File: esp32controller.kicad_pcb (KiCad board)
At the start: 2 copper layers, 80 x 100 mm, 117 parts, among them J1 Conn_02x03_Odd_Even, J10 USB_B_Micro, J11 Conn_01x04_Female, J12 Conn_01x06_Female, J14 Conn_01x04, J15 Conn_01x06, J16 Conn_01x04, J17 Conn_01x04, J18 Conn_01x03, J19 Conn_01x03, J2 Conn_01x04, J20 Conn_01x03, J21 Conn_02x09_Odd_Even, J22 Conn_02x09_Odd_Even, J23 Conn_01x03, J24 Conn_01x03, J25 Conn_01x03, J26 Conn_02x09_Odd_Even, J3 Conn_02x03_Odd_Even, J4 Conn_01x04, J5 Conn_02x03_Odd_Even, J6 Conn_01x04, J7 Micro_SD_Card_Det, J8 Conn_02x03_Odd_Even, J9 Conn_01x04, Q1 Q_NPN_BEC, Q2 Q_NPN_BEC, Q3 Q_NMOS_GDS, Q4 Q_NMOS_GDS, Q5 Q_NMOS_GDS, U1 ESP32-WROOM, U2 CH340C, U3 ADS1015, U4 SX1509, U5 TPS560430, U6 TLV1117-33

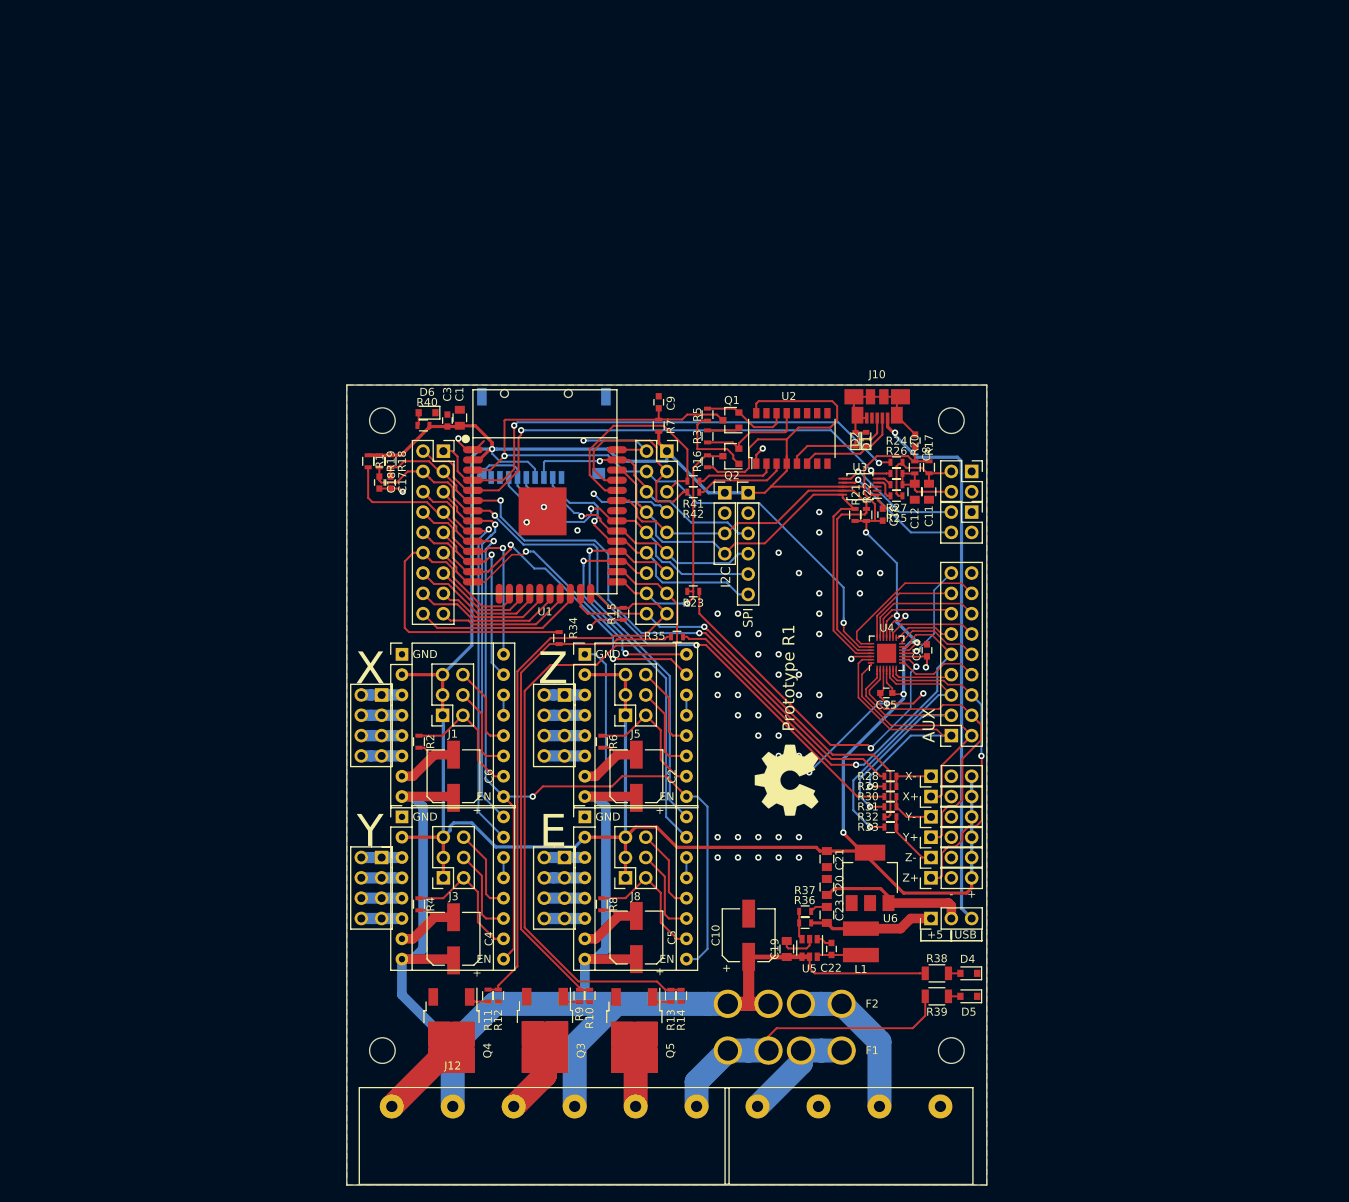
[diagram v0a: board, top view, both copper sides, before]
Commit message: Prototype R2
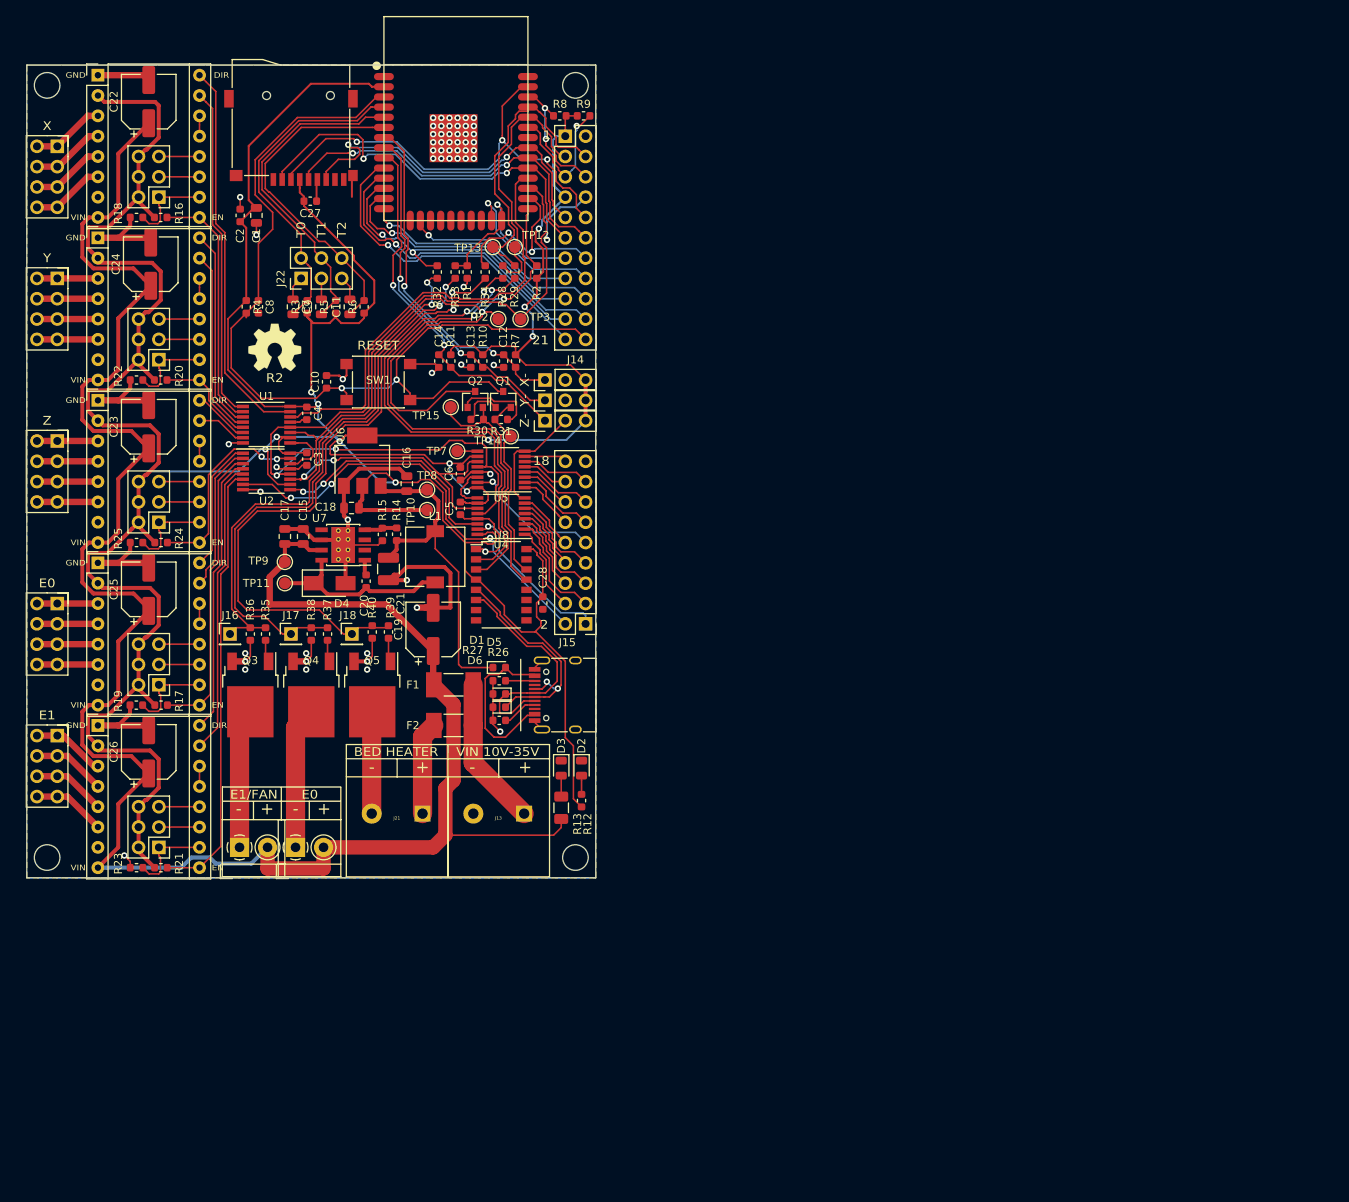
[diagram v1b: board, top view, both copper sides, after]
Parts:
- removed J26: Conn_02x09_Odd_Even, Socket_Strips:Socket_Strip_Straight_2x09_Pitch2.54mm
- removed JP1: Jumper_3_Open, Socket_Strips:Socket_Strip_Straight_1x03_Pitch2.54mm
- removed MK1, MK2, MK3, MK4: Mounting_Hole, Mounting_Holes:MountingHole_3.2mm_M3
- removed R41, R42: 0, Resistors_SMD:R_0603
- removed REF***: OSHW-Symbol_8.9x8mm_SilkScreen, Symbols:OSHW-Symbol_8.9x8mm_SilkScreen
- added A5: Pololu_Breakout_A4988, Module:Pololu_Breakout-16_15.2x20.3mm, F.Cu at (8.89, 82.5)
- added C13: NC, Capacitor_SMD:C_0603_1608Metric, F.Cu at (55.5, 37.0)
- added C24: 100uF, Capacitor_SMD:CP_Elec_6.3x7.7, F.Cu at (15.5, 24.9)
- added C25: 100uF, Capacitor_SMD:CP_Elec_6.3x7.7, F.Cu at (15.2, 65.5)
- added C26: 100uF, Capacitor_SMD:CP_Elec_6.3x7.7, F.Cu at (15.2, 85.9)
- added C27: 100nF, Capacitor_SMD:C_0603_1608Metric, F.Cu at (35.4, 17.0)
- added C28: 100nF, Capacitor_SMD:C_0603_1608Metric, F.Cu at (64.5, 67.2)
- added C7: 10uF, Capacitor_SMD:C_0805_2012Metric, F.Cu at (33.3, 30.2)
- added D3: LED, LED_SMD:LED_0805_2012Metric, F.Cu at (66.8, 87.9)
- added J13: Conn_01x02, ESP32-footprints-Lib:TERM_2-WAY_6.35mm, F.Cu at (59.0, 93.6)
- added REF**: OSHW-Symbol_6.7x6mm_SilkScreen, Symbol:OSHW-Symbol_6.7x6mm_SilkScreen, F.Cu at (31.0, 35.3)
- added REF**: MountingHole_3.2mm_M3_DIN965, MountingHole:MountingHole_3.2mm_M3_DIN965, F.Cu at (68.6, 2.54)
- added REF**: MountingHole_3.2mm_M3_DIN965, MountingHole:MountingHole_3.2mm_M3_DIN965, F.Cu at (2.54, 2.54)
- added REF**: MountingHole_3.2mm_M3_DIN965, MountingHole:MountingHole_3.2mm_M3_DIN965, F.Cu at (2.54, 99.1)
- added REF**: MountingHole_3.2mm_M3_DIN965, MountingHole:MountingHole_3.2mm_M3_DIN965, F.Cu at (68.6, 99.1)
- added SW1: SW_Push, Button_Switch_SMD:SW_Push_1P1T_NO_6x6mm_H9.5mm, F.Cu at (43.9, 39.6)
- added TP10: TestPoint, TestPoint:TestPoint_Pad_D1.5mm, F.Cu at (50.0, 55.6)
- added TP11: TestPoint, TestPoint:TestPoint_Pad_D1.5mm, F.Cu at (32.3, 64.8)
- added TP12: TestPoint, TestPoint:TestPoint_Pad_D1.5mm, F.Cu at (61.0, 22.8)
- added TP13: TestPoint, TestPoint:TestPoint_Pad_D1.5mm, F.Cu at (58.2, 22.8)
- added TP14: TestPoint, TestPoint:TestPoint_Pad_D1.5mm, F.Cu at (60.5, 46.4)
- added TP15: TestPoint, TestPoint:TestPoint_Pad_D1.5mm, F.Cu at (53.0, 42.8)
- added TP2: TestPoint, TestPoint:TestPoint_Pad_D1.5mm, F.Cu at (58.9, 31.8)
- added TP3: TestPoint, TestPoint:TestPoint_Pad_D1.5mm, F.Cu at (61.7, 31.8)
- added TP7: TestPoint, TestPoint:TestPoint_Pad_D1.5mm, F.Cu at (53.8, 48.3)
- added TP8: TestPoint, TestPoint:TestPoint_Pad_D1.5mm, F.Cu at (50.0, 53.1)
- added TP9: TestPoint, TestPoint:TestPoint_Pad_D1.5mm, F.Cu at (32.3, 62.1)
- added U7: TPS5430DDA, Package_SO:TI_SO-PowerPAD-8_ThermalVias, F.Cu at (39.5, 60.0)
- added U8: CH340C, Package_SO:SOP-16_4.4x10.4mm_P1.27mm, F.Cu at (59.3, 65.0)
- C1: value 100uF -> 10uF; footprint Capacitors_SMD:C_0805 -> Capacitor_SMD:C_0805_2012Metric
- C10, C4, C5, C6: value 100uF -> 100nF; footprint Capacitors_SMD:CP_Elec_6.3x7.7 -> Capacitor_SMD:C_0603_1608Metric
- C11: footprint Capacitors_SMD:C_0805 -> Capacitor_SMD:C_0805_2012Metric
- C12: value 10uF -> NC; footprint Capacitors_SMD:C_0805 -> Capacitor_SMD:C_0603_1608Metric
- C14: value 100nF -> NC; footprint Capacitors_SMD:C_0603 -> Capacitor_SMD:C_0603_1608Metric
- C15: value 100nF -> 4.7uF; footprint Capacitors_SMD:C_0603 -> Capacitor_SMD:C_0805_2012Metric
- C16: value 100n -> 10uF; footprint Capacitors_SMD:C_0603 -> Capacitor_SMD:C_0805_2012Metric
- C17: value NC -> 4.7uF; footprint Capacitors_SMD:C_0603 -> Capacitor_SMD:C_0805_2012Metric
- C18: value NC -> 10uF; footprint Capacitors_SMD:C_0603 -> Capacitor_SMD:C_0805_2012Metric
- C19: value 2.2uF -> 100uF; footprint Capacitors_SMD:C_0805 -> Capacitor_SMD:CP_Elec_6.3x7.7
- C2: value 100uF -> 1uF; footprint Capacitors_SMD:CP_Elec_6.3x7.7 -> Capacitor_SMD:C_0603_1608Metric
- C20: value 10uF -> 10nF; footprint Capacitors_SMD:C_0805 -> Capacitor_SMD:C_0603_1608Metric
- C21: value 100uF -> 220uF; footprint Capacitors_SMD:C_0805 -> Capacitor_SMD:C_1210_3225Metric
- C22: value 0.1uF -> 100uF; footprint Capacitors_SMD:C_0603 -> Capacitor_SMD:CP_Elec_6.3x7.7
- C23: value 22uF -> 100uF; footprint Capacitors_SMD:C_0805 -> Capacitor_SMD:CP_Elec_6.3x7.7
- C3: value 1uF -> 100nF; footprint Capacitors_SMD:C_0603 -> Capacitor_SMD:C_0603_1608Metric
- C8: value 100n -> 100nF; footprint Capacitors_SMD:C_0603 -> Capacitor_SMD:C_0603_1608Metric
- C9: value 1nF -> 10uF; footprint Capacitors_SMD:C_0603 -> Capacitor_SMD:C_0805_2012Metric
- D1: value D_TVS -> D_Schottky; footprint Diodes_SMD:D_0603 -> Diode_SMD:D_0603_1608Metric
- D2: value D_TVS -> LED; footprint Diodes_SMD:D_0603 -> LED_SMD:LED_0805_2012Metric
- D4: value LED -> B340A; footprint Diodes_SMD:D_0805 -> Diode_SMD:D_SMA
- D5, D6: value LED -> D_TVS; footprint Diodes_SMD:D_0805 -> Diode_SMD:D_0603_1608Metric
- F1, F2: footprint ESP32Controller:FUSE -> ESP32Controller:Fuse_0679H
- J1, J5: footprint Socket_Strips:Socket_Strip_Straight_2x03_Pitch2.54mm -> Connector_PinHeader_2.54mm:PinHeader_2x03_P2.54mm_Vertical
- J10: value USB_B_Micro -> Conn_01x04; footprint ESP32Controller:473460001 -> ESP32Controller:Socket_Strip_Straight_1x04_Pitch2.54mm_dual
- J11: value Conn_01x04_Female -> Micro_SD_Card_Det; footprint ESP32Controller:KP7.62x4 -> ESP32Controller:microsd
- J12: value Conn_01x06_Female -> USB_C_Receptacle_USB2.0; footprint ESP32Controller:KP7.62x6 -> ESP32Controller:USB_C
- J14: value Conn_01x04 -> Conn_02x11_Odd_Even; footprint Socket_Strips:Socket_Strip_Straight_1x04_Pitch2.54mm -> Connector_PinHeader_2.54mm:PinHeader_2x11_P2.54mm_Vertical
- J15: value Conn_01x06 -> Conn_02x09_Odd_Even; footprint Socket_Strips:Socket_Strip_Straight_1x06_Pitch2.54mm -> Connector_PinHeader_2.54mm:PinHeader_2x09_P2.54mm_Vertical
- J16, J17: value Conn_01x04 -> Conn_01x01; footprint Socket_Strips:Socket_Strip_Straight_2x02_Pitch2.54mm -> Connector_PinHeader_2.54mm:PinHeader_1x01_P2.54mm_Vertical
- J18: value Conn_01x03 -> Conn_01x01; footprint Socket_Strips:Socket_Strip_Straight_1x03_Pitch2.54mm -> Connector_PinHeader_2.54mm:PinHeader_1x01_P2.54mm_Vertical
- J19, J20: value Conn_01x03 -> Conn_01x02; footprint Socket_Strips:Socket_Strip_Straight_1x03_Pitch2.54mm -> TerminalBlock_4Ucon:TerminalBlock_4Ucon_1x02_P3.50mm_Horizontal
- J2, J6, J9: value Conn_01x04 -> Conn_02x03_Odd_Even; footprint ESP32Controller:Socket_Strip_Straight_1x04_Pitch2.54mm_dual -> Connector_PinHeader_2.54mm:PinHeader_2x03_P2.54mm_Vertical
- J21: value Conn_02x09_Odd_Even -> Conn_01x02; footprint Socket_Strips:Socket_Strip_Straight_2x09_Pitch2.54mm -> ESP32-footprints-Lib:TERM_2-WAY_6.35mm
- J22: value Conn_02x09_Odd_Even -> Conn_01x06; footprint Socket_Strips:Socket_Strip_Straight_2x09_Pitch2.54mm -> Connector_PinHeader_2.54mm:PinHeader_2x03_P2.54mm_Vertical
- J23, J24, J25: footprint Socket_Strips:Socket_Strip_Straight_1x03_Pitch2.54mm -> Connector_PinHeader_2.54mm:PinHeader_1x03_P2.54mm_Vertical
- J3, J8: value Conn_02x03_Odd_Even -> Conn_01x04; footprint Socket_Strips:Socket_Strip_Straight_2x03_Pitch2.54mm -> ESP32Controller:Socket_Strip_Straight_1x04_Pitch2.54mm_dual
- J7: value Micro_SD_Card_Det -> Conn_01x04; footprint ESP32Controller:microsd -> ESP32Controller:Socket_Strip_Straight_1x04_Pitch2.54mm_dual; moved to F.Cu
- L1: value 18uH -> 22uH; footprint ESP32Controller:SDR0403 -> Inductor_SMD:L_7.3x7.3_H3.5
- Q1, Q2: footprint TO_SOT_Packages_SMD:SOT-23 -> Package_TO_SOT_SMD:SOT-23
- Q3, Q4, Q5: footprint TO_SOT_Packages_SMD:TO-252-2 -> Package_TO_SOT_SMD:TO-252-2
- R1: value 10k -> DNP 10k; footprint Resistors_SMD:R_0603 -> Resistor_SMD:R_0603_1608Metric
- R10, R14, R2, R4: value 100k -> 10k; footprint Resistors_SMD:R_0603 -> Resistor_SMD:R_0603_1608Metric
- R11: value 10 -> 10k; footprint Resistors_SMD:R_0603 -> Resistor_SMD:R_0603_1608Metric
- R12: value 100k -> R; footprint Resistors_SMD:R_0603 -> Resistor_SMD:R_0603_1608Metric
- R13: value 10 -> 2.4k; footprint Resistors_SMD:R_0603 -> Resistor_SMD:R_1206_3216Metric
- R15: value 5k -> 3.24k; footprint Resistors_SMD:R_0603 -> Resistor_SMD:R_0603_1608Metric
- R16: value 5k -> 10k; footprint Resistors_SMD:R_0603 -> Resistor_SMD:R_0603_1608Metric
- R17, R20, R21: value 4.7k -> 10k; footprint Resistors_SMD:R_0603 -> Resistor_SMD:R_0603_1608Metric
- R18, R19: value 10k -> 100k; footprint Resistors_SMD:R_0603 -> Resistor_SMD:R_0603_1608Metric
- R22: value 4.7k -> 100k; footprint Resistors_SMD:R_0603 -> Resistor_SMD:R_0603_1608Metric
- R23, R25: value 0 -> 100k; footprint Resistors_SMD:R_0603 -> Resistor_SMD:R_0603_1608Metric
- R24, R30, R31: value 0 -> 10k; footprint Resistors_SMD:R_0603 -> Resistor_SMD:R_0603_1608Metric
- R26, R27: value 0 -> 5.1k; footprint Resistors_SMD:R_0603 -> Resistor_SMD:R_0603_1608Metric
- R28, R32, R33, R34: footprint Resistors_SMD:R_0603 -> Resistor_SMD:R_0603_1608Metric
- R29: value 0 -> 499; footprint Resistors_SMD:R_0603 -> Resistor_SMD:R_0603_1608Metric
- R3, R5: value 12k -> 4.7k; footprint Resistors_SMD:R_0603 -> Resistor_SMD:R_0603_1608Metric
- R35: value 0 -> 10; footprint Resistors_SMD:R_0603 -> Resistor_SMD:R_0603_1608Metric
- R36: value 88.7k -> 100k; footprint Resistors_SMD:R_0603 -> Resistor_SMD:R_0603_1608Metric
- R37: value 22.1k -> 10; footprint Resistors_SMD:R_0603 -> Resistor_SMD:R_0603_1608Metric
- R38: value 1.5k -> 100k; footprint Resistors_SMD:R_1206 -> Resistor_SMD:R_0603_1608Metric
- R39: value 1.5k -> 10; footprint Resistors_SMD:R_1206 -> Resistor_SMD:R_0603_1608Metric
- R40: value R -> 100k; footprint Resistors_SMD:R_0603 -> Resistor_SMD:R_0603_1608Metric
- R6, R8: value 100k -> 4.7k; footprint Resistors_SMD:R_0603 -> Resistor_SMD:R_0603_1608Metric
- R7: value 12k -> 10k; footprint Resistors_SMD:R_0603 -> Resistor_SMD:R_0603_1608Metric
- R9: value 10 -> 4.7k; footprint Resistors_SMD:R_0603 -> Resistor_SMD:R_0603_1608Metric
- U1: value ESP32-WROOM -> 74HC595; footprint ESP32-footprints-Lib:ESP32-WROOM -> Package_SO:TSSOP-16_4.4x5mm_P0.65mm
- U2: value CH340C -> 74HC595; footprint Housings_SSOP:SOP-16_4.4x10.4mm_Pitch1.27mm -> Package_SO:TSSOP-16_4.4x5mm_P0.65mm
- U3: value ADS1015 -> ESP32-WROOM; footprint Housings_SSOP:TSSOP-10_3x3mm_Pitch0.5mm -> ESP32-footprints-Lib:ESP32-WROOM
- U4: value SX1509 -> 74HC595; footprint Housings_DFN_QFN:QFN-28-1EP_4x4mm_Pitch0.4mm -> Package_SO:TSSOP-16_4.4x5mm_P0.65mm
- U5: value TPS560430 -> 74HC595; footprint TO_SOT_Packages_SMD:SOT-23-6 -> Package_SO:TSSOP-16_4.4x5mm_P0.65mm
- U6: footprint TO_SOT_Packages_SMD:SOT-223-3_TabPin2 -> Package_TO_SOT_SMD:SOT-223-3_TabPin2
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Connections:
- A1 pad 15: /IO27 -> Q1
- A1 pad 16: /IO26 -> Q0
- A1 pad 2: VCC -> +3.3V
- A1 pad 8: +24V -> VIN_FUSED
- A1 pad 9: /IO25 -> Q2
- A2 pad 15: /IO33 -> Q4
- A2 pad 16: /IO32 -> Q3
- A2 pad 2: VCC -> +3.3V
- A2 pad 8: +24V -> VIN_FUSED
- A2 pad 9: /IO25 -> Q5
- A3 pad 15: /IO14 -> Q7
- A3 pad 16: /IO12 -> Q6
- A3 pad 2: VCC -> +3.3V
- A3 pad 8: +24V -> VIN_FUSED
- A3 pad 9: /IO25 -> Q8
- A4 pad 15: /E0_STEP -> Q10
- A4 pad 16: /E0_DIR -> Q9
- A4 pad 2: VCC -> +3.3V
- A4 pad 8: +24V -> VIN_FUSED
- A4 pad 9: /IO25 -> Q11
- C1 pad 1: VCC -> +3.3V
- C10 pad 1: +24V -> EN
- C11 pad 1: /THERM0 -> THERM2
- C12 pad 1: /THERM1 -> X_MIN
- C14 pad 1: VCC -> Z_MIN
- C15 pad 1: VCC -> VIN_FUSED
- C16 pad 1: VCC -> +5V
- C17 pad 1: /IO34 -> VIN_FUSED
- C18 pad 1: /IO35 -> +3.3V
- C19 pad 1: +24V -> VIN_FUSED
- C2 pad 1: +24V -> +3.3V
- C20 pad 2: GND -> Net-(C20-Pad2)
- C21 pad 1: VCC -> +5V
- C22 pad 1: Net-(C22-Pad1) -> VIN_FUSED
- C22 pad 2: Net-(C22-Pad2) -> GND
- C23 pad 1: +5V -> VIN_FUSED
- C3 pad 1: VCC -> +3.3V
- C4 pad 1: +24V -> +3.3V
- C5 pad 1: +24V -> +3.3V
- C6 pad 1: +24V -> +3.3V
- C8 pad 1: VCC -> EN
- C9 pad 1: /EN -> THERM1
- D1 pad 1: Net-(D1-Pad1) -> +5V
- D1 pad 2: GND -> VBUS
- D2 pad 1: Net-(D2-Pad1) -> GND
- D2 pad 2: GND -> Net-(D2-Pad2)
- D4 pad 1: GND -> Net-(C20-Pad1)
- D4 pad 2: Net-(D4-Pad2) -> GND
- D5 pad 1: GND -> Net-(D5-Pad1)
- D5 pad 2: Net-(D5-Pad2) -> GND
- D6 pad 1: GND -> Net-(D6-Pad1)
- D6 pad 2: Net-(D6-Pad2) -> GND
- F1 pad 1: /+24V2 -> VIN_FUSED
- F1 pad 2: Net-(F1-Pad2) -> VIN
- F2 pad 1: +24V -> VBED_FUSED
- F2 pad 2: Net-(F2-Pad2) -> VIN
- J1 pad 1: VCC -> Net-(A1-Pad10)
- J1 pad 2: Net-(A1-Pad10) -> +3.3V
- J1 pad 3: VCC -> Net-(A1-Pad11)
- J1 pad 4: Net-(A1-Pad11) -> +3.3V
- J1 pad 5: VCC -> Net-(A1-Pad12)
- J1 pad 6: Net-(A1-Pad12) -> +3.3V
- J10 pad 1: VBUS -> Net-(A3-Pad3)
- J10 pad 2: Net-(D2-Pad1) -> Net-(A3-Pad4)
- J10 pad 3: Net-(D1-Pad1) -> Net-(A3-Pad5)
- J10 pad 4: (no net) -> Net-(A3-Pad6)
- J11 pad 1: Net-(F1-Pad2) -> (no net)
- J11 pad 2: GND -> VSPI_SS
- J11 pad 3: Net-(F2-Pad2) -> VSPI_MOSI
- J11 pad 4: GND -> +3.3V
- J14 pad 1: VCC -> +3.3V
- J14 pad 3: /IO21 -> RXD
- J14 pad 4: /IO22 -> TXD
- J15 pad 1: VCC -> Q16
- J15 pad 2: GND -> Q15
- J15 pad 3: /IO23 -> Q18
- J15 pad 4: /IO18 -> Q17
- J15 pad 5: /IO19 -> Q20
- J15 pad 6: /IO5 -> Q19
- J16 pad 1: GND -> FAN_IN
- J17 pad 1: GND -> HEATER_IN
- J18 pad 1: /X_MIN -> BED_IN
- J19 pad 1: /Y_MIN -> FAN_OUT
- J19 pad 2: GND -> VIN_FUSED
- J2 pad 1: Net-(A1-Pad3) -> Net-(A4-Pad10)
- J2 pad 2: Net-(A1-Pad4) -> +3.3V
- J2 pad 3: Net-(A1-Pad5) -> Net-(A4-Pad11)
- J2 pad 4: Net-(A1-Pad6) -> +3.3V
- J20 pad 1: /Z_MIN -> HEATER_OUT
- J20 pad 2: GND -> VIN_FUSED
- J21 pad 1: /SVP -> VBED_FUSED
- J21 pad 2: /SVN -> BED_OUT
- J22 pad 1: VCC -> GND
- J22 pad 2: GND -> THERM0
- J22 pad 3: /TXD -> GND
- J22 pad 4: /EN -> THERM1
- J22 pad 5: /RXD -> GND
- J22 pad 6: /IO23 -> THERM2
- J23 pad 1: /XIO1 -> X_MIN
- J23 pad 3: VCC -> +3.3V
- J24 pad 1: /XIO3 -> Y_MIN
- J24 pad 3: VCC -> +3.3V
- J25 pad 1: /XIO5 -> Z_MIN
- J25 pad 3: VCC -> +3.3V
- J3 pad 1: VCC -> Net-(A1-Pad3)
- J3 pad 2: Net-(A2-Pad10) -> Net-(A1-Pad4)
- J3 pad 3: VCC -> Net-(A1-Pad5)
- J3 pad 4: Net-(A2-Pad11) -> Net-(A1-Pad6)
- J4 pad 1: Net-(A2-Pad3) -> Net-(A4-Pad3)
- J4 pad 2: Net-(A2-Pad4) -> Net-(A4-Pad4)
- J4 pad 3: Net-(A2-Pad5) -> Net-(A4-Pad5)
- J4 pad 4: Net-(A2-Pad6) -> Net-(A4-Pad6)
- J5 pad 1: VCC -> Net-(A2-Pad10)
- J5 pad 2: Net-(A3-Pad10) -> +3.3V
- J5 pad 3: VCC -> Net-(A2-Pad11)
- J5 pad 4: Net-(A3-Pad11) -> +3.3V
- J5 pad 5: VCC -> Net-(A2-Pad12)
- J5 pad 6: Net-(A3-Pad12) -> +3.3V
- J6 pad 1: Net-(A3-Pad3) -> Net-(A5-Pad10)
- J6 pad 2: Net-(A3-Pad4) -> +3.3V
- J6 pad 3: Net-(A3-Pad5) -> Net-(A5-Pad11)
- J6 pad 4: Net-(A3-Pad6) -> +3.3V
- J7 pad 1: (no net) -> Net-(A2-Pad3)
- J7 pad 2: /IO5 -> Net-(A2-Pad4)
- J7 pad 3: /IO23 -> Net-(A2-Pad5)
- J7 pad 4: VCC -> Net-(A2-Pad6)
- J8 pad 1: VCC -> Net-(A5-Pad3)
- J8 pad 2: Net-(A4-Pad10) -> Net-(A5-Pad4)
- J8 pad 3: VCC -> Net-(A5-Pad5)
- J8 pad 4: Net-(A4-Pad11) -> Net-(A5-Pad6)
- J9 pad 1: Net-(A4-Pad3) -> Net-(A3-Pad10)
- J9 pad 2: Net-(A4-Pad4) -> +3.3V
- J9 pad 3: Net-(A4-Pad5) -> Net-(A3-Pad11)
- J9 pad 4: Net-(A4-Pad6) -> +3.3V
- L1 pad 1: Net-(C22-Pad2) -> Net-(C20-Pad1)
- Q1 pad 2: /RTS -> RTS
- Q1 pad 3: /EN -> EN
- Q2 pad 2: /DTR -> DTR
- Q2 pad 3: /IO0 -> BCLK
- Q3 pad 2: /FAN_OUT -> FAN_OUT
- Q4 pad 2: /HEATER_OUT -> HEATER_OUT
- Q5 pad 2: /BED_OUT -> BED_OUT
- R1 pad 1: VCC -> GND
- R1 pad 2: /IO25 -> HEATER
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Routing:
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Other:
- board size 80 x 100 mm -> 71.1 x 101.6 mm
- board text added: "1"
- board text added: "18"
- board text added: "2"
- board text added: "21"
- board text added: "BED HEATER"
- board text added: "DIR"
- board text added: "E0"
- board text added: "E1"
- board text added: "E1/FAN"
- board text added: "R2"
- board text added: "RESET"
- board text added: "T0"
- board text added: "T1"
- board text added: "T2"
- board text added: "VIN"
- board text added: "VIN 10V-35V"
- board text removed: "+5"
- board text removed: "AUX"
- board text removed: "E"
- board text removed: "I2C"
- board text removed: "Prototype R1"
- board text removed: "SPI"
- board text removed: "USB"
- board text removed: "X+"
- board text removed: "Y+"
- board text removed: "Z+"

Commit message: Prototype R3
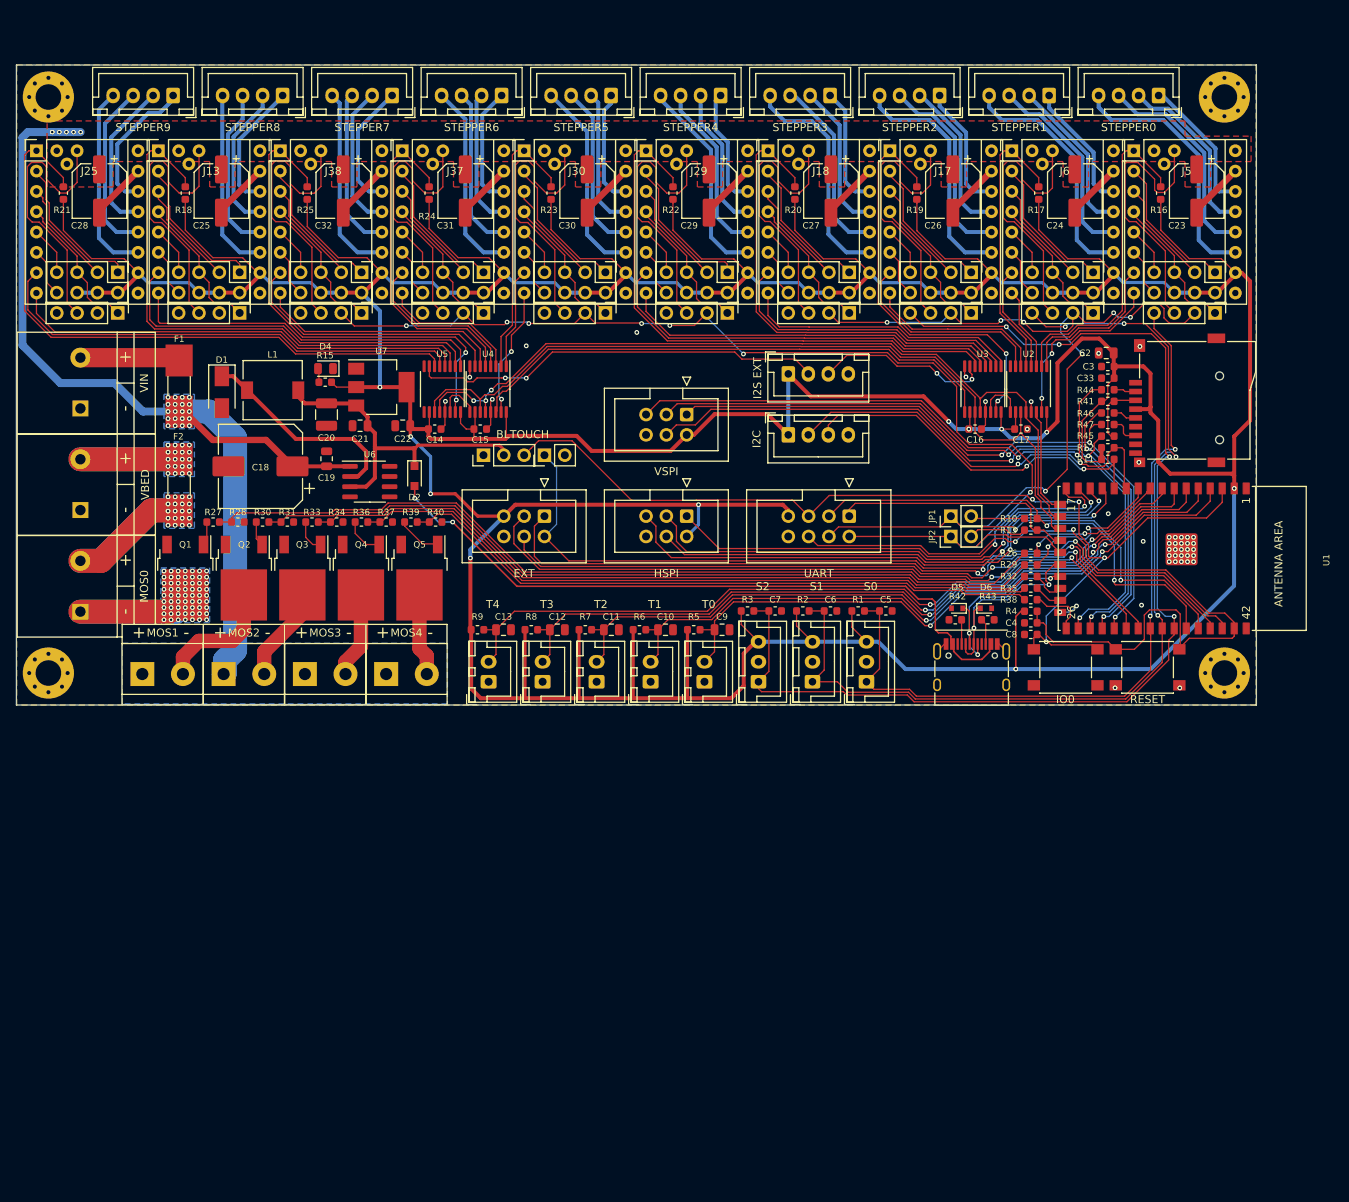
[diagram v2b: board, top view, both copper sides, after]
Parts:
- removed A1, A2, A3, A4, A5: Pololu_Breakout_A4988, Module:Pololu_Breakout-16_15.2x20.3mm
- removed C1: 10uF, Capacitor_SMD:C_0805_2012Metric
- removed D3: LED, LED_SMD:LED_0805_2012Metric
- removed R14: 10k, Resistor_SMD:R_0603_1608Metric
- removed the REF** at (31.0, 35.3)
- removed the REF** at (68.6, 2.54)
- removed the REF** at (2.54, 2.54)
- removed the REF** at (2.54, 99.1)
- removed the REF** at (68.6, 99.1)
- removed TP10, TP11, TP12, TP13, TP14, TP15, TP2, TP3, TP7, TP8, TP9: TestPoint, TestPoint:TestPoint_Pad_D1.5mm
- removed U8: CH340C, Package_SO:SOP-16_4.4x10.4mm_P1.27mm
- added C29: 100uF/35V, Capacitor_SMD:CP_Elec_6.3x7.7, F.Cu at (85.3, 15.7)
- added C30: 100uF/35V, Capacitor_SMD:CP_Elec_6.3x7.7, F.Cu at (70.0, 15.7)
- added C31: 100uF/35V, Capacitor_SMD:CP_Elec_6.3x7.7, F.Cu at (54.8, 15.7)
- added C32: 100uF/35V, Capacitor_SMD:CP_Elec_6.3x7.7, F.Cu at (39.6, 15.7)
- added C33: 100nF, Capacitor_SMD:C_0603_1608Metric, F.Cu at (135.1, 39.1)
- added J26: STEPPER9, Connector_JST:JST_XH_B4B-XH-A_1x04_P2.50mm_Vertical, F.Cu at (18.3, 3.81)
- added J27: Conn_02x04_Odd_Even, Connector_PinHeader_2.54mm:PinHeader_2x04_P2.54mm_Vertical, F.Cu at (87.6, 25.9)
- added J28: Conn_02x04_Odd_Even, Connector_PinHeader_2.54mm:PinHeader_2x04_P2.54mm_Vertical, F.Cu at (72.3, 25.9)
- added J29: TMC2209, ESP32Controller:pololu, F.Cu at (84.0, 19.6)
- added J30: TMC2209, ESP32Controller:pololu, F.Cu at (68.8, 19.6)
- added J31: STEPPER4, Connector_JST:JST_XH_B4B-XH-A_1x04_P2.50mm_Vertical, F.Cu at (86.7, 3.81)
- added J32: STEPPER5, Connector_JST:JST_XH_B4B-XH-A_1x04_P2.50mm_Vertical, F.Cu at (73.0, 3.81)
- added J33: Conn_02x02_Odd_Even, Connector_PinHeader_2.54mm:PinHeader_1x04_P2.54mm_Vertical, F.Cu at (57.1, 31.0)
- added J34: Conn_02x02_Odd_Even, Connector_PinHeader_2.54mm:PinHeader_1x04_P2.54mm_Vertical, F.Cu at (41.8, 31.0)
- added J35: Conn_02x04_Odd_Even, Connector_PinHeader_2.54mm:PinHeader_2x04_P2.54mm_Vertical, F.Cu at (57.1, 25.9)
- added J36: Conn_02x04_Odd_Even, Connector_PinHeader_2.54mm:PinHeader_2x04_P2.54mm_Vertical, F.Cu at (41.8, 25.9)
- added J37: TMC2209, ESP32Controller:pololu, F.Cu at (53.5, 19.6)
- added J38: TMC2209, ESP32Controller:pololu, F.Cu at (38.3, 19.6)
- added J39: STEPPER6, Connector_JST:JST_XH_B4B-XH-A_1x04_P2.50mm_Vertical, F.Cu at (59.4, 3.81)
- added J40: STEPPER7, Connector_JST:JST_XH_B4B-XH-A_1x04_P2.50mm_Vertical, F.Cu at (45.7, 3.81)
- added J41: T0, Connector_JST:JST_XH_B2B-XH-A_1x02_P2.50mm_Vertical, F.Cu at (84.7, 77.1)
- added J42: HSPI, Connector_IDC:IDC-Header_2x03_P2.54mm_Vertical, F.Cu at (82.5, 56.4)
- added J43: I2S EXT, Connector_JST:JST_XH_B4B-XH-A_1x04_P2.50mm_Vertical, F.Cu at (95.2, 38.6)
- added J44: UART, Connector_IDC:IDC-Header_2x04_P2.54mm_Vertical, F.Cu at (102.8, 56.4)
- added J45: S0, Connector_JST:JST_XH_B3B-XH-A_1x03_P2.50mm_Vertical, F.Cu at (105.0, 77.1)
- added J46: T1, Connector_JST:JST_XH_B2B-XH-A_1x02_P2.50mm_Vertical, F.Cu at (78.0, 77.1)
- added J47: VIN, ESP32-footprints-Lib:TERM_2-WAY_6.35mm, F.Cu at (6.70, 39.8)
- added J48: T2, Connector_JST:JST_XH_B2B-XH-A_1x02_P2.50mm_Vertical, F.Cu at (71.2, 77.1)
- added J49: S1, Connector_JST:JST_XH_B3B-XH-A_1x03_P2.50mm_Vertical, F.Cu at (98.2, 77.1)
- added J50: VSPI, Connector_IDC:IDC-Header_2x03_P2.54mm_Vertical, F.Cu at (82.5, 43.7)
- added J51: T3, Connector_JST:JST_XH_B2B-XH-A_1x02_P2.50mm_Vertical, F.Cu at (64.5, 77.1)
- added J52: S2, Connector_JST:JST_XH_B3B-XH-A_1x03_P2.50mm_Vertical, F.Cu at (91.5, 77.1)
- added J53: I2C, Connector_JST:JST_XH_B4B-XH-A_1x04_P2.50mm_Vertical, F.Cu at (95.2, 46.2)
- added J54: T4, Connector_JST:JST_XH_B2B-XH-A_1x02_P2.50mm_Vertical, F.Cu at (57.7, 77.1)
- added J55: BLTOUCH, Connector_PinHeader_2.54mm:PinHeader_1x03_P2.54mm_Vertical, F.Cu at (57.1, 48.8)
- added J56: EXT, Connector_IDC:IDC-Header_2x03_P2.54mm_Vertical, F.Cu at (64.7, 56.4)
- added J57: Conn_01x02, Connector_PinHeader_2.54mm:PinHeader_1x02_P2.54mm_Vertical, F.Cu at (64.7, 48.8)
- added J59: MOS0, ESP32-footprints-Lib:TERM_2-WAY_6.35mm, F.Cu at (6.70, 65.2)
- added J61: MOS1, TerminalBlock:TerminalBlock_bornier-2_P5.08mm, F.Cu at (14.4, 76.1)
- added J64: MOS2, TerminalBlock:TerminalBlock_bornier-2_P5.08mm, F.Cu at (24.6, 76.1)
- added J66: MOS3, TerminalBlock:TerminalBlock_bornier-2_P5.08mm, F.Cu at (34.8, 76.1)
- added J67: USB_C_Receptacle_USB2.0, ESP32Controller:USB_C, F.Cu at (118.1, 77.5)
- added J68: Micro_SD_Card_Det, ESP32Controller:microsd, F.Cu at (149.1, 41.9)
- added J69: MOS4, TerminalBlock:TerminalBlock_bornier-2_P5.08mm, F.Cu at (44.9, 76.1)
- added J70: VBED, ESP32-footprints-Lib:TERM_2-WAY_6.35mm, F.Cu at (6.70, 52.5)
- added JP1: Jumper, Connector_PinHeader_2.54mm:PinHeader_1x02_P2.54mm_Vertical, F.Cu at (115.5, 56.4)
- added JP2: Jumper, Connector_PinHeader_2.54mm:PinHeader_1x02_P2.54mm_Vertical, F.Cu at (115.5, 58.9)
- added R41: 10k, Resistor_SMD:R_0603_1608Metric, F.Cu at (135.1, 42.0)
- added R42: 5.1k, Resistor_SMD:R_0603_1608Metric, F.Cu at (116.1, 69.3)
- added R43: 5.1k, Resistor_SMD:R_0603_1608Metric, F.Cu at (120.1, 69.3)
- added R44: 220, Resistor_SMD:R_0603_1608Metric, F.Cu at (135.1, 40.6)
- added R45: 220, Resistor_SMD:R_0603_1608Metric, F.Cu at (135.1, 46.4)
- added R46: 220, Resistor_SMD:R_0603_1608Metric, F.Cu at (135.1, 43.5)
- added R47: 220, Resistor_SMD:R_0603_1608Metric, F.Cu at (135.1, 44.9)
- added REF**: MountingHole_3.2mm_M3_Pad_Via, MountingHole:MountingHole_3.2mm_M3_Pad_Via, F.Cu at (149.7, 76.0)
- added REF**: MountingHole_3.2mm_M3_Pad_Via, MountingHole:MountingHole_3.2mm_M3_Pad_Via, F.Cu at (2.70, 76.0)
- added REF**: MountingHole_3.2mm_M3_Pad_Via, MountingHole:MountingHole_3.2mm_M3_Pad_Via, F.Cu at (2.70, 4.00)
- added REF**: MountingHole_3.2mm_M3_Pad_Via, MountingHole:MountingHole_3.2mm_M3_Pad_Via, F.Cu at (149.7, 4.00)
- added SW2: IO0, Button_Switch_SMD:SW_Push_1P1T_NO_6x6mm_H9.5mm, F.Cu at (129.9, 75.3)
- C10: value 100nF -> 10uF; footprint Capacitor_SMD:C_0603_1608Metric -> Capacitor_SMD:C_0805_2012Metric
- C12, C13: value NC -> 10uF; footprint Capacitor_SMD:C_0603_1608Metric -> Capacitor_SMD:C_0805_2012Metric
- C14: value NC -> 100nF
- C15, C17: value 4.7uF -> 100nF; footprint Capacitor_SMD:C_0805_2012Metric -> Capacitor_SMD:C_0603_1608Metric
- C16: value 10uF -> 100nF; footprint Capacitor_SMD:C_0805_2012Metric -> Capacitor_SMD:C_0603_1608Metric
- C18: value 10uF -> 470uF/35V; footprint Capacitor_SMD:C_0805_2012Metric -> Capacitor_SMD:CP_Elec_10x10
- C19: value 100uF -> 4.7uF/35V; footprint Capacitor_SMD:CP_Elec_6.3x7.7 -> Capacitor_SMD:C_0805_2012Metric
- C2: value 1uF -> 22uF; footprint Capacitor_SMD:C_0603_1608Metric -> Capacitor_SMD:C_0805_2012Metric
- C20: value 10nF -> 220uF/35V; footprint Capacitor_SMD:C_0603_1608Metric -> Capacitor_SMD:C_1210_3225Metric
- C21: value 220uF -> 10uF; footprint Capacitor_SMD:C_1210_3225Metric -> Capacitor_SMD:C_0805_2012Metric
- C22: value 100uF -> 10uF; footprint Capacitor_SMD:CP_Elec_6.3x7.7 -> Capacitor_SMD:C_0805_2012Metric
- C23, C24, C25, C26: value 100uF -> 100uF/35V
- C27, C28: value 100nF -> 100uF/35V; footprint Capacitor_SMD:C_0603_1608Metric -> Capacitor_SMD:CP_Elec_6.3x7.7
- C5, C6: value 100nF -> NC
- C7: value 10uF -> NC; footprint Capacitor_SMD:C_0805_2012Metric -> Capacitor_SMD:C_0603_1608Metric
- D1: value D_Schottky -> B340A; footprint Diode_SMD:D_0603_1608Metric -> Diode_SMD:D_SMA
- D2: value LED -> D_Schottky; footprint LED_SMD:LED_0805_2012Metric -> Diode_SMD:D_SOD-323_HandSoldering
- D4: value B340A -> LED; footprint Diode_SMD:D_SMA -> LED_SMD:LED_0805_2012Metric
- D5, D6: footprint Diode_SMD:D_0603_1608Metric -> Diode_SMD:D_SOD-523
- F1, F2: footprint ESP32Controller:Fuse_0679H -> ESP32Controller:Fuse_holder_0679H
- J1, J2, J9: value Conn_02x03_Odd_Even -> Conn_02x02_Odd_Even; footprint Connector_PinHeader_2.54mm:PinHeader_2x03_P2.54mm_Vertical -> Connector_PinHeader_2.54mm:PinHeader_1x04_P2.54mm_Vertical
- J10: value Conn_01x04 -> Conn_02x02_Odd_Even; footprint ESP32Controller:Socket_Strip_Straight_1x04_Pitch2.54mm_dual -> Connector_PinHeader_2.54mm:PinHeader_1x04_P2.54mm_Vertical
- J11: value Micro_SD_Card_Det -> Conn_02x02_Odd_Even; footprint ESP32Controller:microsd -> Connector_PinHeader_2.54mm:PinHeader_1x04_P2.54mm_Vertical
- J12: value USB_C_Receptacle_USB2.0 -> Conn_02x04_Odd_Even; footprint ESP32Controller:USB_C -> Connector_PinHeader_2.54mm:PinHeader_2x04_P2.54mm_Vertical
- J13: value Conn_01x02 -> TMC2209; footprint ESP32-footprints-Lib:TERM_2-WAY_6.35mm -> ESP32Controller:pololu
- J14: value Conn_02x11_Odd_Even -> STEPPER8; footprint Connector_PinHeader_2.54mm:PinHeader_2x11_P2.54mm_Vertical -> Connector_JST:JST_XH_B4B-XH-A_1x04_P2.50mm_Vertical
- J15: value Conn_02x09_Odd_Even -> Conn_02x04_Odd_Even; footprint Connector_PinHeader_2.54mm:PinHeader_2x09_P2.54mm_Vertical -> Connector_PinHeader_2.54mm:PinHeader_2x04_P2.54mm_Vertical
- J16: value Conn_01x01 -> Conn_02x04_Odd_Even; footprint Connector_PinHeader_2.54mm:PinHeader_1x01_P2.54mm_Vertical -> Connector_PinHeader_2.54mm:PinHeader_2x04_P2.54mm_Vertical
- J17, J18: value Conn_01x01 -> TMC2209; footprint Connector_PinHeader_2.54mm:PinHeader_1x01_P2.54mm_Vertical -> ESP32Controller:pololu
- J19: value Conn_01x02 -> STEPPER2; footprint TerminalBlock_4Ucon:TerminalBlock_4Ucon_1x02_P3.50mm_Horizontal -> Connector_JST:JST_XH_B4B-XH-A_1x04_P2.50mm_Vertical
- J20: value Conn_01x02 -> STEPPER3; footprint TerminalBlock_4Ucon:TerminalBlock_4Ucon_1x02_P3.50mm_Horizontal -> Connector_JST:JST_XH_B4B-XH-A_1x04_P2.50mm_Vertical
- J21: value Conn_01x02 -> Conn_02x02_Odd_Even; footprint ESP32-footprints-Lib:TERM_2-WAY_6.35mm -> Connector_PinHeader_2.54mm:PinHeader_1x04_P2.54mm_Vertical
- J22: value Conn_01x06 -> Conn_02x04_Odd_Even; footprint Connector_PinHeader_2.54mm:PinHeader_2x03_P2.54mm_Vertical -> Connector_PinHeader_2.54mm:PinHeader_2x04_P2.54mm_Vertical
- J23, J24: value Conn_01x03 -> Conn_02x02_Odd_Even; footprint Connector_PinHeader_2.54mm:PinHeader_1x03_P2.54mm_Vertical -> Connector_PinHeader_2.54mm:PinHeader_1x04_P2.54mm_Vertical
- J25: value Conn_01x03 -> TMC2209; footprint Connector_PinHeader_2.54mm:PinHeader_1x03_P2.54mm_Vertical -> ESP32Controller:pololu
- J3, J4: value Conn_01x04 -> Conn_02x04_Odd_Even; footprint ESP32Controller:Socket_Strip_Straight_1x04_Pitch2.54mm_dual -> Connector_PinHeader_2.54mm:PinHeader_2x04_P2.54mm_Vertical
- J5, J6: value Conn_02x03_Odd_Even -> TMC2209; footprint Connector_PinHeader_2.54mm:PinHeader_2x03_P2.54mm_Vertical -> ESP32Controller:pololu
- J7: value Conn_01x04 -> STEPPER0; footprint ESP32Controller:Socket_Strip_Straight_1x04_Pitch2.54mm_dual -> Connector_JST:JST_XH_B4B-XH-A_1x04_P2.50mm_Vertical
- J8: value Conn_01x04 -> STEPPER1; footprint ESP32Controller:Socket_Strip_Straight_1x04_Pitch2.54mm_dual -> Connector_JST:JST_XH_B4B-XH-A_1x04_P2.50mm_Vertical
- L1: value 22uH -> 68uH
- Q1, Q2: value Q_NPN_BEC -> Q_NMOS_GDS; footprint Package_TO_SOT_SMD:SOT-23 -> Package_TO_SOT_SMD:TO-252-2
- R1: value DNP 10k -> 10k
- R10: value 10k -> 1k
- R11, R7: value 10k -> 4.7k
- R12: value R -> 4.7k
- R13: value 2.4k -> 1k; footprint Resistor_SMD:R_1206_3216Metric -> Resistor_SMD:R_0603_1608Metric
- R15: value 3.24k -> R
- R18, R19, R22, R23, R25: value 100k -> 10k
- R26: value 5.1k -> 0
- R27: value 5.1k -> 10
- R28, R34: value 0 -> 100k
- R29: value 499 -> 0
- R3: value 4.7k -> 10k
- R30: value 10k -> 10
- R31: value 10k -> 100k
- R33: value 0 -> 10
- R35: value 10 -> 0
- R36: value 100k -> 10
- R37: value 10 -> 100k
- R38: value 100k -> 0
- SW1: value SW_Push -> RESET
- U1: value 74HC595 -> ESP32-S2-WROOM; footprint Package_SO:TSSOP-16_4.4x5mm_P0.65mm -> ESP32Controller:esp32-s2-wrooom
- U3: value ESP32-WROOM -> 74HC595; footprint ESP32-footprints-Lib:ESP32-WROOM -> Package_SO:TSSOP-16_4.4x5mm_P0.65mm
- U6: value TLV1117-33 -> XL1509; footprint Package_TO_SOT_SMD:SOT-223-3_TabPin2 -> Package_SO:SOIC-8_3.9x4.9mm_P1.27mm
- U7: value TPS5430DDA -> TLV1117-33; footprint Package_SO:TI_SO-PowerPAD-8_ThermalVias -> Package_TO_SOT_SMD:SOT-223-3_TabPin2
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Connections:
- C10 pad 1: EN -> THERM1
- C12 pad 1: X_MIN -> THERM3
- C13 pad 1: Y_MIN -> THERM4
- C14 pad 1: Z_MIN -> +3.3V
- C15 pad 1: VIN_FUSED -> +3.3V
- C16 pad 1: +5V -> +3.3V
- C17 pad 1: VIN_FUSED -> +3.3V
- C18 pad 1: +3.3V -> VIN_FUSED
- C20 pad 1: Net-(C20-Pad1) -> +5V
- C20 pad 2: Net-(C20-Pad2) -> GND
- C22 pad 1: VIN_FUSED -> +3.3V
- C27 pad 1: +3.3V -> VIN_FUSED
- C28 pad 1: +3.3V -> VIN_FUSED
- C4 pad 1: +3.3V -> EN
- C5 pad 1: +3.3V -> S0_MIN
- C6 pad 1: +3.3V -> S1_MIN
- C7 pad 1: GND -> S2_MIN
- C7 pad 2: THERM0 -> GND
- C8 pad 1: EN -> IO0
- C9 pad 1: THERM1 -> GND
- C9 pad 2: GND -> THERM0
- D1 pad 1: +5V -> Net-(D1-Pad1)
- D1 pad 2: VBUS -> GND
- D2 pad 1: GND -> +5V
- D2 pad 2: Net-(D2-Pad2) -> VBUS
- D4 pad 1: Net-(C20-Pad1) -> GND
- D4 pad 2: GND -> Net-(D4-Pad2)
- D5 pad 1: Net-(D5-Pad1) -> USB_D+
- D6 pad 1: Net-(D6-Pad1) -> USB_D-
- F2 pad 2: VIN -> VBED
- J1 pad 1: Net-(A1-Pad10) -> Net-(J1-Pad1)
- J1 pad 2: +3.3V -> RX0
- J1 pad 3: Net-(A1-Pad11) -> Net-(J1-Pad3)
- J1 pad 4: +3.3V -> S0_MIN
- J10 pad 1: Net-(A3-Pad3) -> Net-(J10-Pad1)
- J10 pad 2: Net-(A3-Pad4) -> RX0
- J10 pad 3: Net-(A3-Pad5) -> Net-(J10-Pad3)
- J10 pad 4: Net-(A3-Pad6) -> S2_MIN
- J11 pad 1: (no net) -> Net-(J11-Pad1)
- J11 pad 2: VSPI_SS -> RX0
- J11 pad 3: VSPI_MOSI -> Net-(J11-Pad3)
- J11 pad 4: +3.3V -> GND
- J13 pad 1: VIN -> Q27
- J13 pad 2: GND -> Net-(J12-Pad1)
- J14 pad 1: +3.3V -> Net-(J13-Pad14)
- J14 pad 2: GND -> Net-(J13-Pad13)
- J14 pad 3: RXD -> Net-(J13-Pad12)
- J14 pad 4: TXD -> Net-(J13-Pad11)
- J15 pad 1: Q16 -> Net-(J15-Pad1)
- J15 pad 2: Q15 -> +3.3V
- J15 pad 3: Q18 -> Net-(J15-Pad3)
- J15 pad 4: Q17 -> +3.3V
- J15 pad 5: Q20 -> Net-(J10-Pad1)
- J15 pad 6: Q19 -> +3.3V
- J15 pad 7: Q22 -> Net-(J15-Pad7)
- J15 pad 8: Q21 -> Net-(J15-Pad8)
- J16 pad 1: FAN_IN -> Net-(J16-Pad1)
- J17 pad 1: HEATER_IN -> Q8
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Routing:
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- added copper zone on B.Cu, net MOS0_OUT
- added copper zone on B.Cu, net VBED
- added copper zone on B.Cu, net VBED_FUSED
- added copper zone on B.Cu, net VIN_FUSED
- added copper zone on F.Cu, net VIN_FUSED
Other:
- board size 71.1 x 101.6 mm -> 155 x 80 mm
- net class Default: trace_width 0.25 -> 0.15; via_dia 0.8 -> 0.6; via_drill 0.4 -> 0.3
- rule trace_min: 0.2 -> 0.15
- rule via_min_size: 0.4 -> 0.6
- board text added: "3.3V"
- board text added: "5V"
- board text added: "CLK"
- board text added: "CS"
- board text added: "DIAG"
- board text added: "IO0"
- board text added: "IO38"
- board text added: "IO39"
- board text added: "IO45"
- board text added: "IO46"
- board text added: "LPBK"
- board text added: "MISO"
- board text added: "MOS0"
- board text added: "MOS1"
- board text added: "MOS2"
- board text added: "MOS3"
- board text added: "MOS4"
- board text added: "MOSI"
- board text added: "MS1"
- board text added: "MS2"
- board text added: "MS3"
- board text added: "PDN"
- board text added: "Q15"
- board text added: "Q31"
- board text added: "RST"
- board text added: "RX0"
- board text added: "RX1"
- board text added: "S0"
- board text added: "S1"
- board text added: "S2"
- board text added: "SCL"
- board text added: "SDA"
- board text added: "SLP"
- board text added: "T3"
- board text added: "T4"
- board text added: "TX0"
- board text added: "TX1"
- board text added: "V3.3"
- board text added: "VBED"
- board text removed: "1"
- board text removed: "18"
- board text removed: "2"
- board text removed: "21"
- board text removed: "BED HEATER"
- board text removed: "DIR"
- board text removed: "E0"
- board text removed: "E1"
- board text removed: "E1/FAN"
- board text removed: "R2"
- board text removed: "RESET"
- board text removed: "VIN 10V-35V"
- board text removed: "X"
- board text removed: "X-"
- board text removed: "Y"
- board text removed: "Y-"
- board text removed: "Z"
- board text removed: "Z-"
